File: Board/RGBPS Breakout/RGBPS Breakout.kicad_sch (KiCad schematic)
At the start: 10 parts, among them IC1 APDS-9999, J1 Conn_01x04_Pin

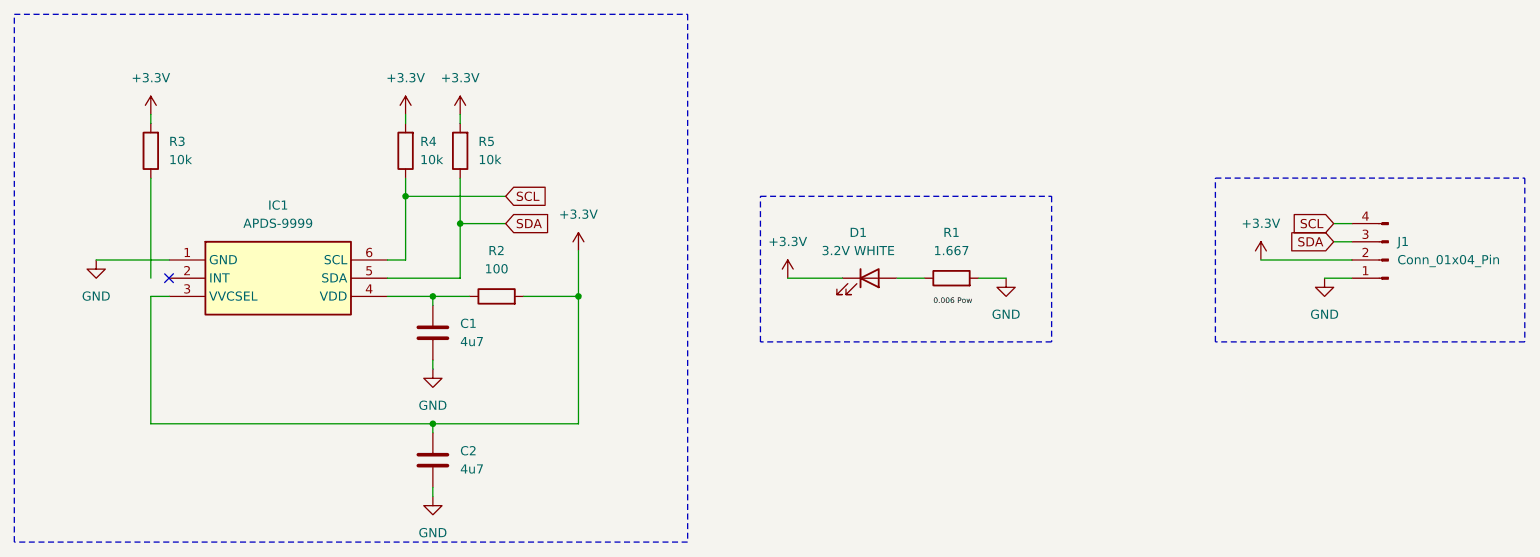
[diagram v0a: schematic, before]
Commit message: interrupt pin
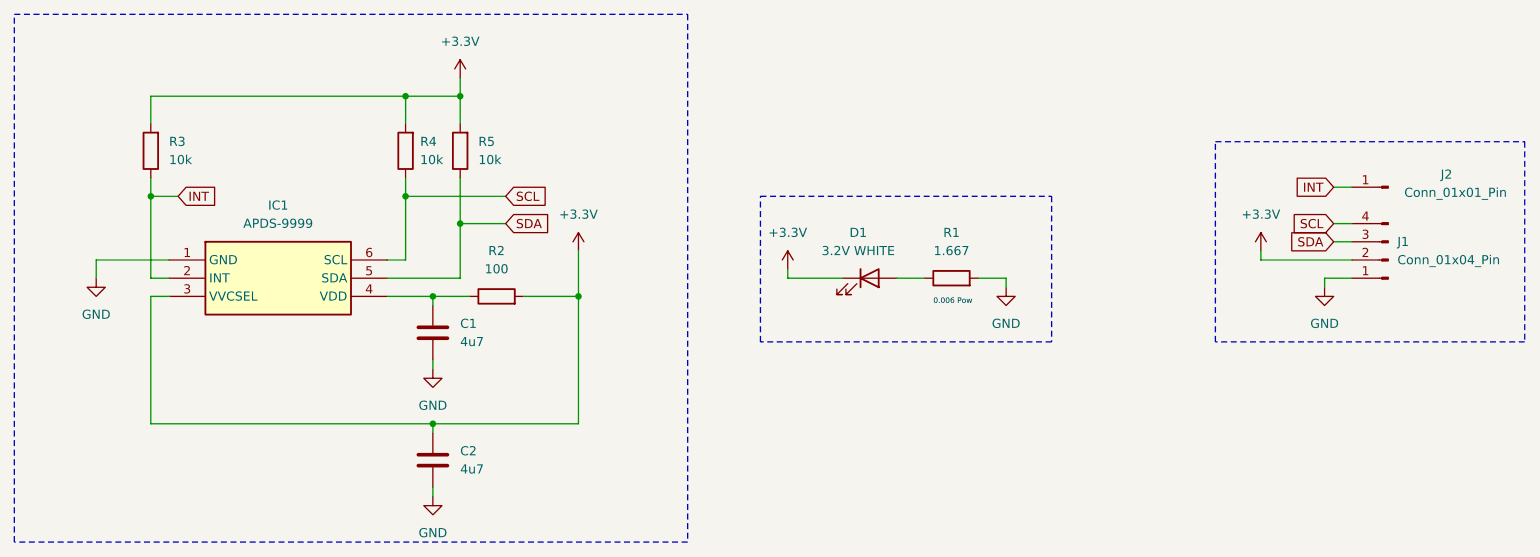
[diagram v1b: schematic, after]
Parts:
- added J2: Conn_01x01_Pin, symbol Connector:Conn_01x01_Pin
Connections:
- net INT: now reaches IC1.2 (INT)
- net INT: now also R3.1, J2.1 (Pin_1)
- no-connect marks 1 -> 0
